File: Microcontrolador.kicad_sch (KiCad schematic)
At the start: 9 parts, among them IC1 AT89LS51-16AU, J2 68000-106HLF

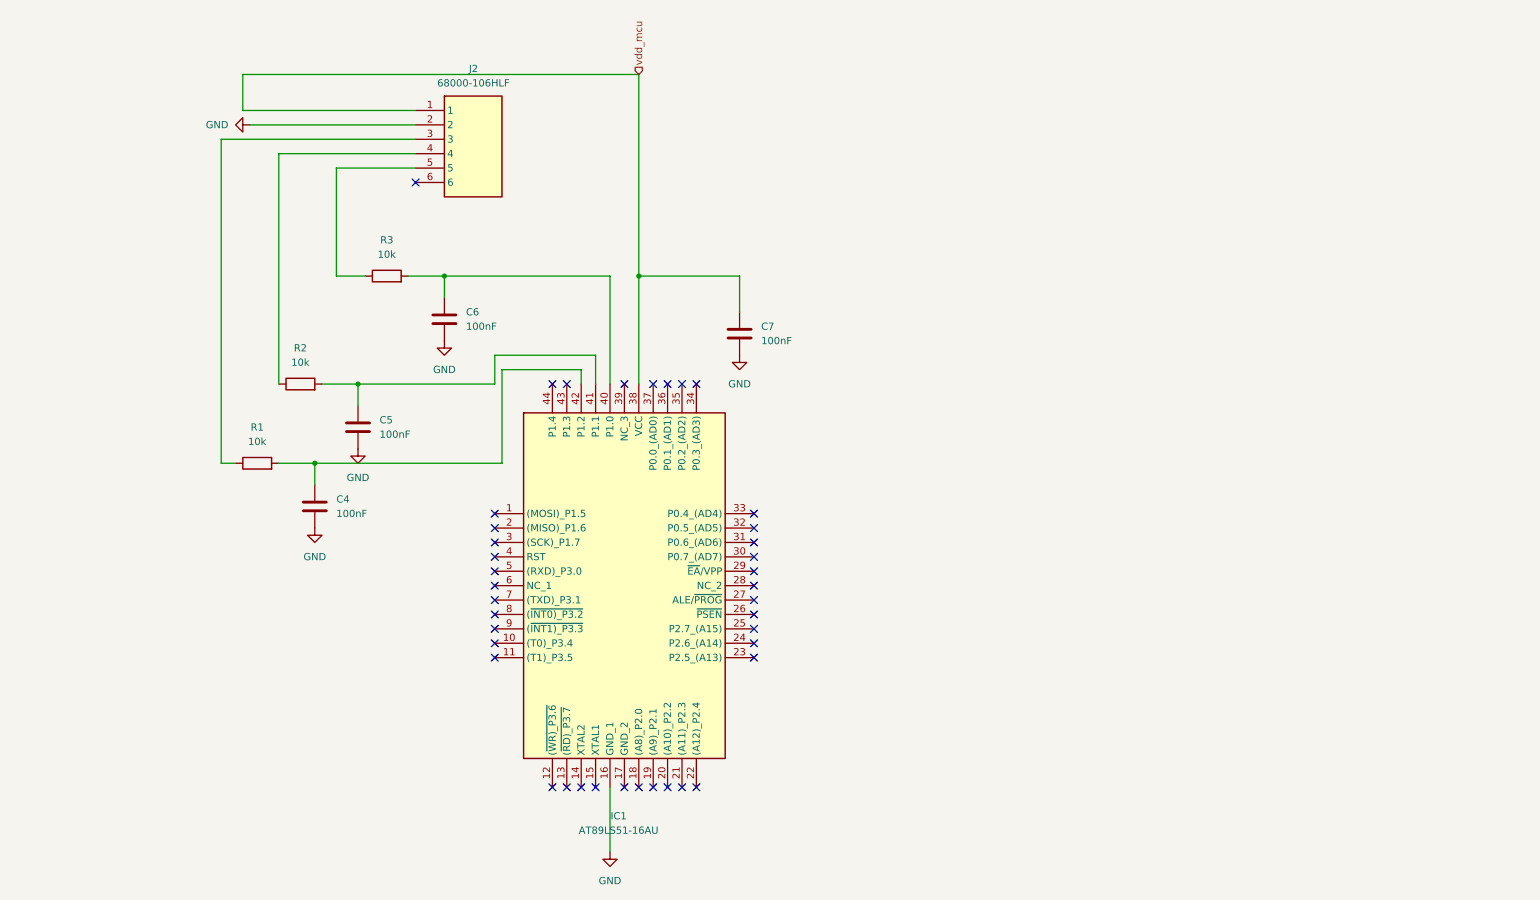
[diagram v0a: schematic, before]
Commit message: sesion 4
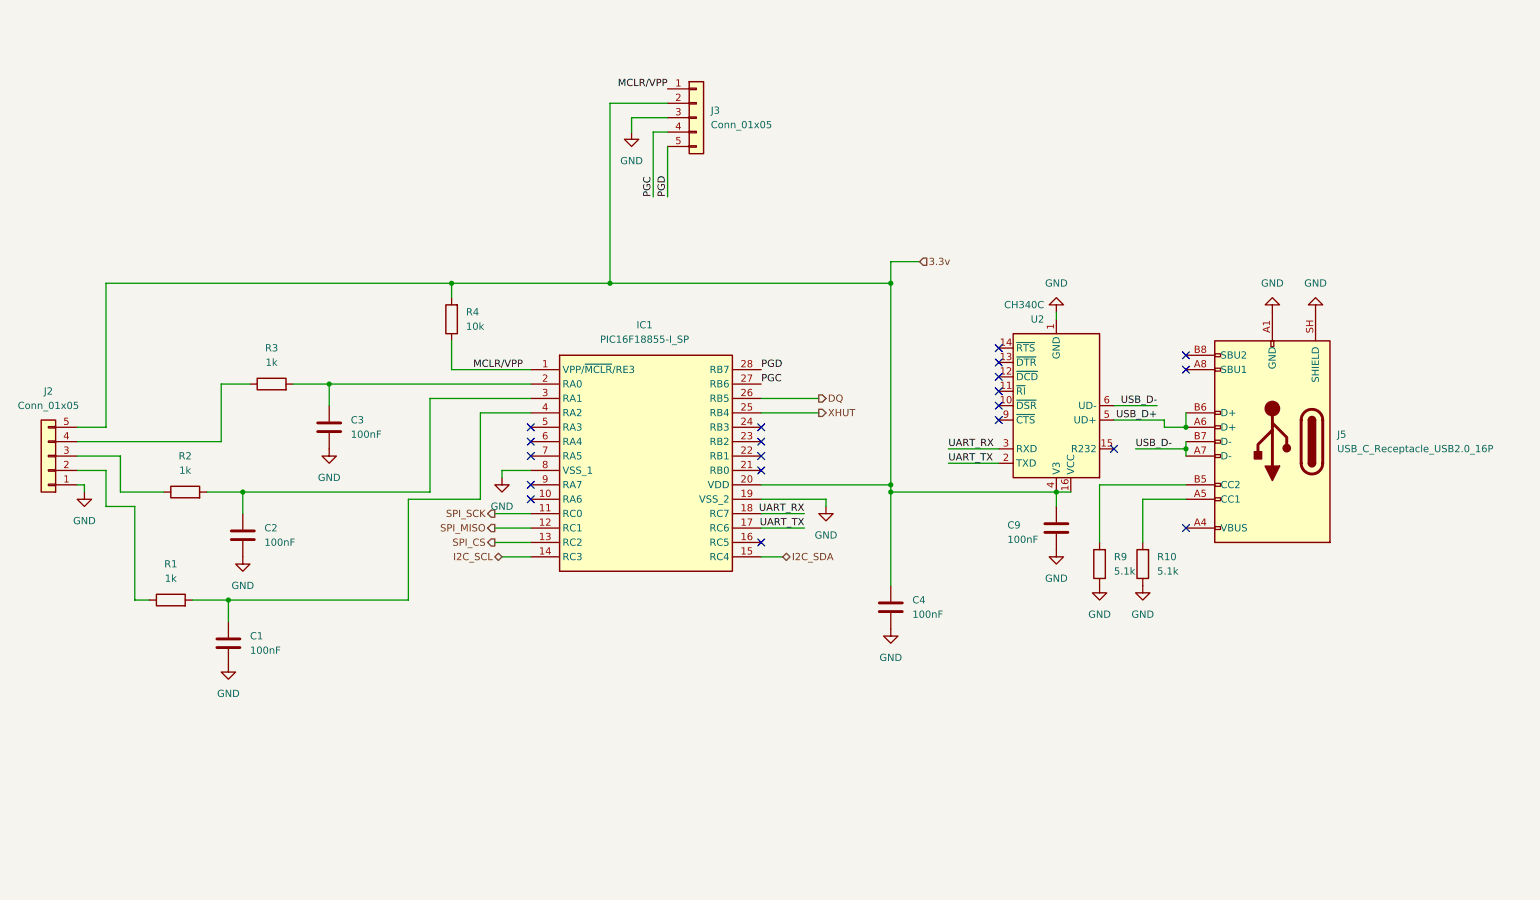
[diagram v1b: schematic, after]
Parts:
- removed C7: 100nF, Capacitor_SMD:C_0402_1005Metric, symbol Device:C
- removed IC1: AT89LS51-16AU, Samacsys:QFP80P1200X1200X120-44N, symbol Samacsys:AT89LS51-16AU
- removed J2: 68000-106HLF, Samacsys:HDRV6W64P0X254_1X6_1524X254X839P, symbol Samacsys:68000-106HLF
- added C4, C9: 100nF, Capacitor_SMD:C_0402_1005Metric, symbol Device:C
- added IC1: PIC16F18855-I_SP, Samacsys:DIP794W56P254L3486H508Q28N, symbol Samacsys:PIC16F18855-I_SP
- added J2, J3: Conn_01x05, Connector_PinHeader_2.54mm:PinHeader_1x05_P2.54mm_Vertical, symbol Connector_Generic:Conn_01x05
- added J5: USB_C_Receptacle_USB2.0_16P, Connector_USB:USB_C_Receptacle_GCT_USB4105-xx-A_16P_TopMnt_Horizontal, symbol Connector:USB_C_Receptacle_USB2.0_16P
- added R10, R9: 5.1k, Resistor_SMD:R_0402_1005Metric_Pad0.72x0.64mm_HandSolder, symbol Device:R
- added R4: 10k, Resistor_SMD:R_0402_1005Metric_Pad0.72x0.64mm_HandSolder, symbol Device:R
- added U2: CH340C, Package_SO:SOIC-16_3.9x9.9mm_P1.27mm, symbol Interface_USB:CH340C
- R1, R2, R3: value 10k -> 1k
- renumbered C4 to C1, C5 to C2, C6 to C3
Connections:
- net GND: now also C4.2, C9.2, IC1.19 (VSS_2), IC1.8 (VSS_1), J2.1 (Pin_1), J3.3 (Pin_3), J5.A1 (GND), J5.A12 (GND), J5.B1 (GND), J5.B12 (GND), J5.SH (SHIELD), R10.1, R9.1, U2.1 (GND)
- net at R2.1: now also J2.3 (Pin_3)
- net at C2.1, R2.2: now also IC1.3 (RA1)
- net at C3.1, R3.2: now also IC1.2 (RA0)
- net at C1.1, R1.2: now also IC1.4 (RA2)
- net at R1.1: now also J2.2 (Pin_2)
- net at R3.1: now also J2.4 (Pin_4)
- new net: J5.A4 (VBUS), J5.A9 (VBUS), J5.B4 (VBUS), J5.B9 (VBUS)
- new net: J5.A5 (CC1), R10.2
- new net: J5.B5 (CC2), R9.2
- new net 3.3v: C4.1, C9.1, IC1.20 (VDD), J2.5 (Pin_5), J3.2 (Pin_2), R4.2, U2.16 (VCC), U2.4 (V3)
- new net DQ: IC1.26 (RB5)
- new net I2C_SCL: IC1.14 (RC3)
- new net I2C_SDA: IC1.15 (RC4)
- new net MCLR/VPP: IC1.1 (VPP/~{MCLR}/RE3), J3.1 (Pin_1), R4.1
- new net PGC: IC1.27 (RB6), J3.4 (Pin_4)
- new net PGD: IC1.28 (RB7), J3.5 (Pin_5)
- new net SPI_CS: IC1.13 (RC2)
- new net SPI_MISO: IC1.12 (RC1)
- new net SPI_SCK: IC1.11 (RC0)
- new net UART_RX: IC1.18 (RC7), U2.3 (RXD)
- new net UART_TX: IC1.17 (RC6), U2.2 (TXD)
- new net USB_D+: J5.A6 (D+), J5.B6 (D+), U2.5 (UD+)
- new net USB_D-: J5.A7 (D-), J5.B7 (D-), U2.6 (UD-)
- new net XHUT: IC1.25 (RB4)
- no-connect marks 40 -> 20
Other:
- moved on the sheet: C1, C2, C3, R1, R2, R3
